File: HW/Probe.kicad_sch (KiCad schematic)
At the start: 33 parts, among them U1 NUCLEO-L432KC

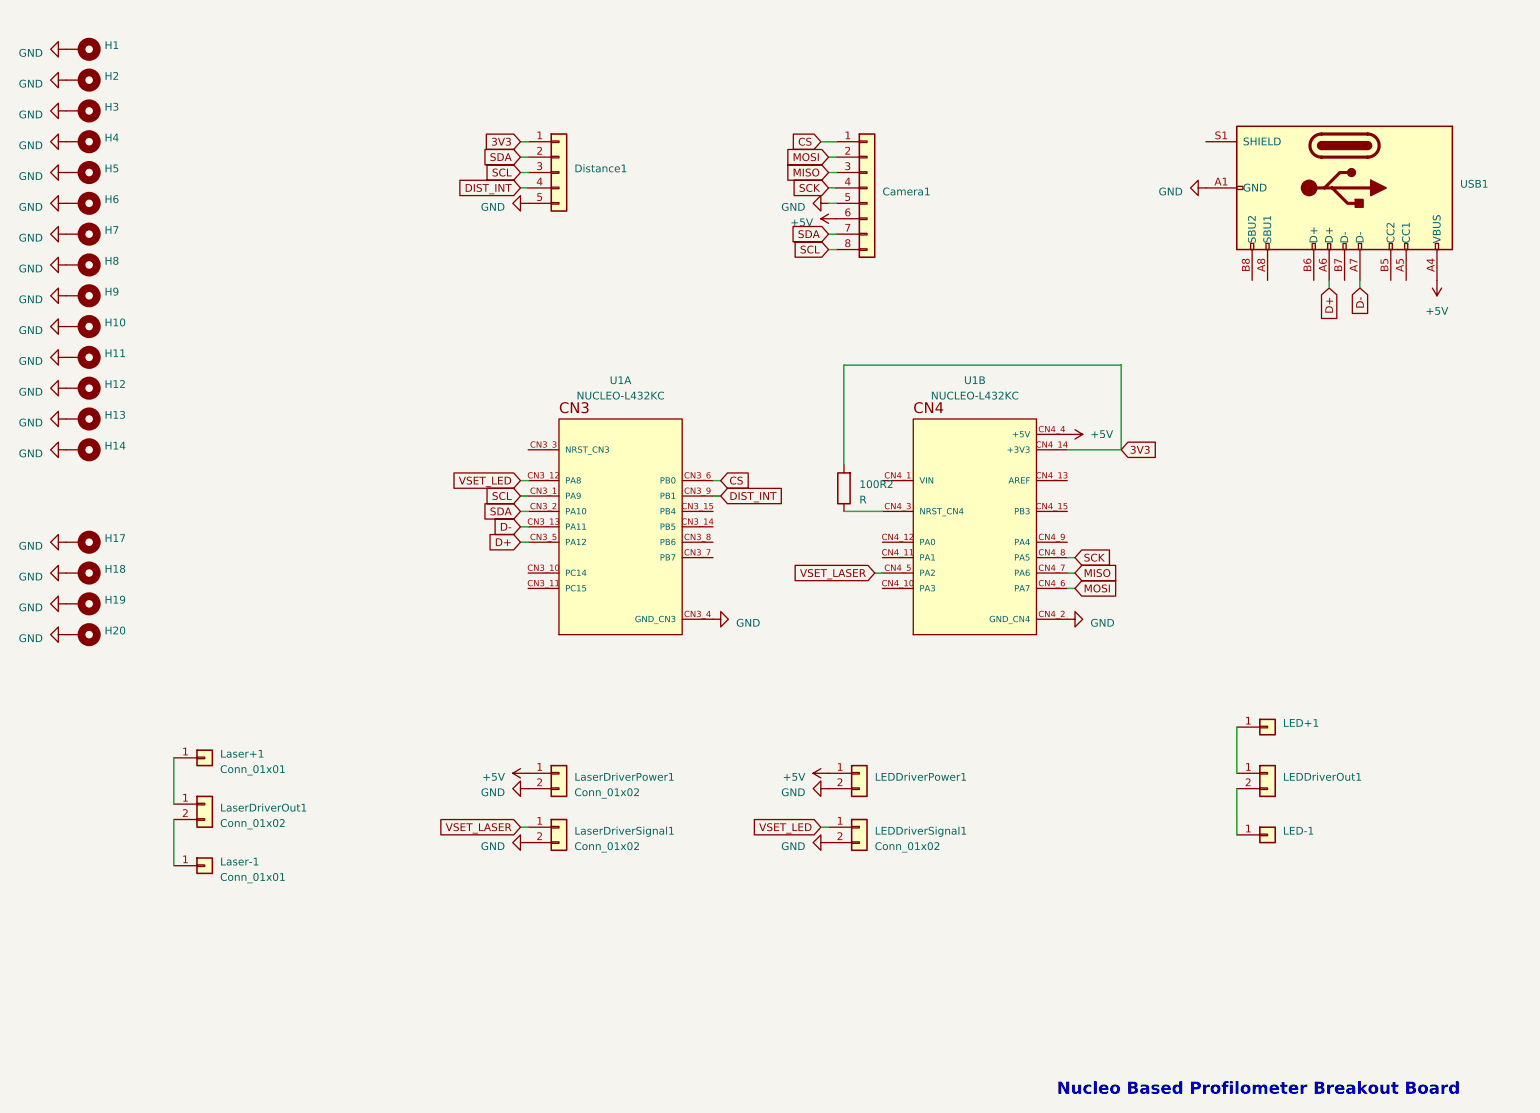
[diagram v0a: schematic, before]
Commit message: Update PCB
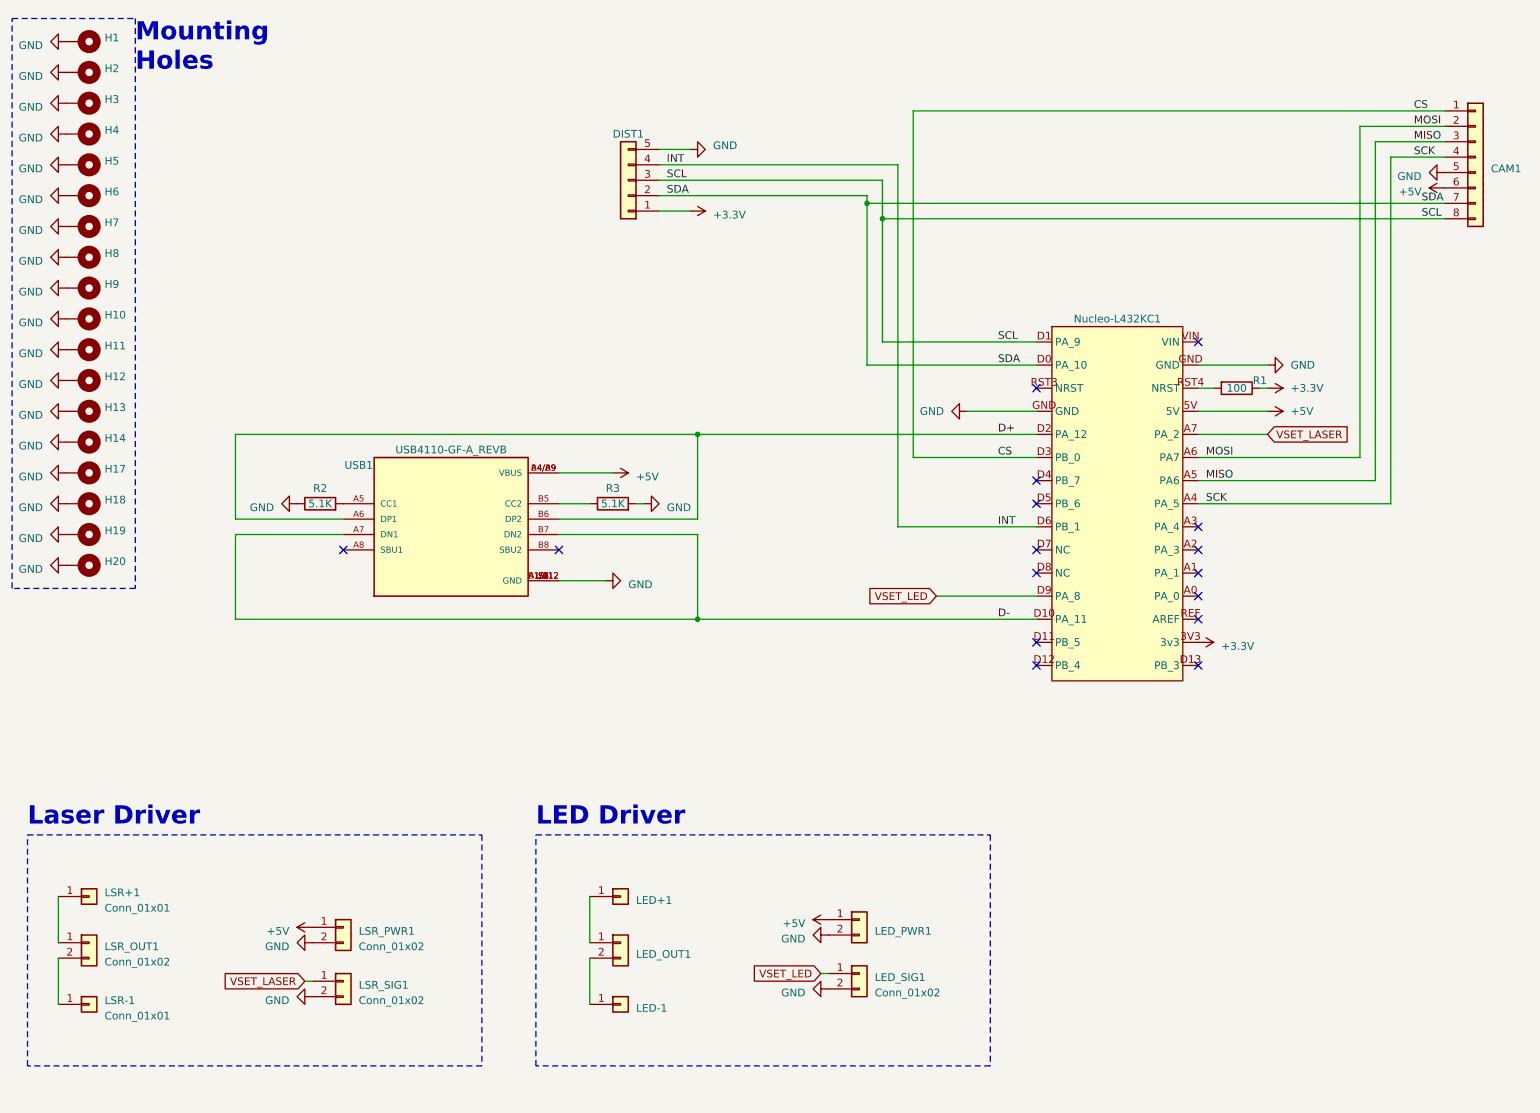
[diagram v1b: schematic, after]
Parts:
- removed 100R2: R, Resistor_SMD:R_0603_1608Metric, symbol Device:R
- removed U1: NUCLEO-L432KC, MODULE_NUCLEO-L432KC, symbol NUCLEO-L432KC:NUCLEO-L432KC
- removed USB1: USB_C_Receptacle_USB2.0, KiCad:2171820001, symbol Connector:USB_C_Receptacle_USB2.0
- added Nucleo-L432KC1: ~, Library:MODULE_NUCLEO-L432KC, symbol Custom_Symbols:Nucleo-L432KC
- added R1: 100, Resistor_SMD:R_0603_1608Metric, symbol Device:R
- added R2, R3: 5.1K, Resistor_SMD:R_0603_1608Metric, symbol Device:R
- added USB1: USB4110-GF-A_REVB, GCT_USB4110-GF-A_REVB, symbol USB4110-GF-A_REVB:USB4110-GF-A_REVB
- CAM1: renamed from Camera1; footprint Connector_PinHeader_1.27mm:PinHeader_1x08_P1.27mm_Vertical -> Connector_PinSocket_2.54mm:PinSocket_1x08_P2.54mm_Vertical
- DIST1: renamed from Distance1; footprint Connector_PinHeader_1.27mm:PinHeader_1x05_P1.27mm_Vertical -> Connector_PinSocket_2.54mm:PinSocket_1x05_P2.54mm_Vertical
- H1, H10, H11, H12, H13, H14, H17, H18, H19, H2, H20, H3, H4, H5, H6, H7, H8, H9: footprint MountingHole:MountingHole_3.2mm_M3_Pad -> MountingHole:MountingHole_3.2mm_M3_Pad_Via
- renumbered LEDDriverOut1 to LED_OUT1, LEDDriverPower1 to LED_PWR1, LEDDriverSignal1 to LED_SIG1, Laser+1 to LSR+1, Laser-1 to LSR-1, LaserDriverOut1 to LSR_OUT1, LaserDriverPower1 to LSR_PWR1, LaserDriverSignal1 to LSR_SIG1
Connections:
- net +5V: now also Nucleo-L432KC1.5V, USB1.A4/B9 (VBUS), USB1.B4/A9 (VBUS)
- net CS: now also Nucleo-L432KC1.D3 (PB_0)
- net D+: now also Nucleo-L432KC1.D2 (PA_12), USB1.A6 (DP1), USB1.B6 (DP2)
- net D-: now also Nucleo-L432KC1.D10 (PA_11), USB1.A7 (DN1), USB1.B7 (DN2)
- net GND: now also Nucleo-L432KC1.GND, R2.1, R3.2, USB1.A1/B12 (GND), USB1.B1/A12 (GND), USB1.S1 (GND), USB1.S2 (GND), USB1.S3 (GND), USB1.S4 (GND)
- net MISO: now also Nucleo-L432KC1.A5 (PA6)
- net MOSI: now also Nucleo-L432KC1.A6 (PA7)
- net SCK: now also Nucleo-L432KC1.A4 (PA_5)
- net SCL: now also Nucleo-L432KC1.D1 (PA_9)
- net SDA: now also Nucleo-L432KC1.D0 (PA_10)
- net VSET_LASER: now also Nucleo-L432KC1.A7 (PA_2)
- net VSET_LED: now also Nucleo-L432KC1.D9 (PA_8)
- net 3V3 renamed +3.3V
- net +3.3V: now also Nucleo-L432KC1.3V3 (3v3), R1.1
- net DIST_INT renamed INT
- net INT: now also Nucleo-L432KC1.D6 (PB_1)
- new net: Nucleo-L432KC1.RST4 (NRST), R1.2
- new net: R2.2, USB1.A5 (CC1)
- new net: R3.1, USB1.B5 (CC2)
- no-connect marks 0 -> 16
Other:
- note added: "LED Driver"
- note added: "Laser Driver"
- note added: "Mounting Holes"
- note removed: "Nucleo Based Profilometer Breakout Board"
- moved on the sheet: CAM1, DIST1, H1, H10, H11, H12, H13, H14, H17, H18, H19, H2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
